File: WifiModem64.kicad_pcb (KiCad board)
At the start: 2 copper layers, 4 parts, among them J1 C64-UserPort, J2 PWR1, U1 WeMos_mini, U2 WeMos_D1_mini_OLED_Shield

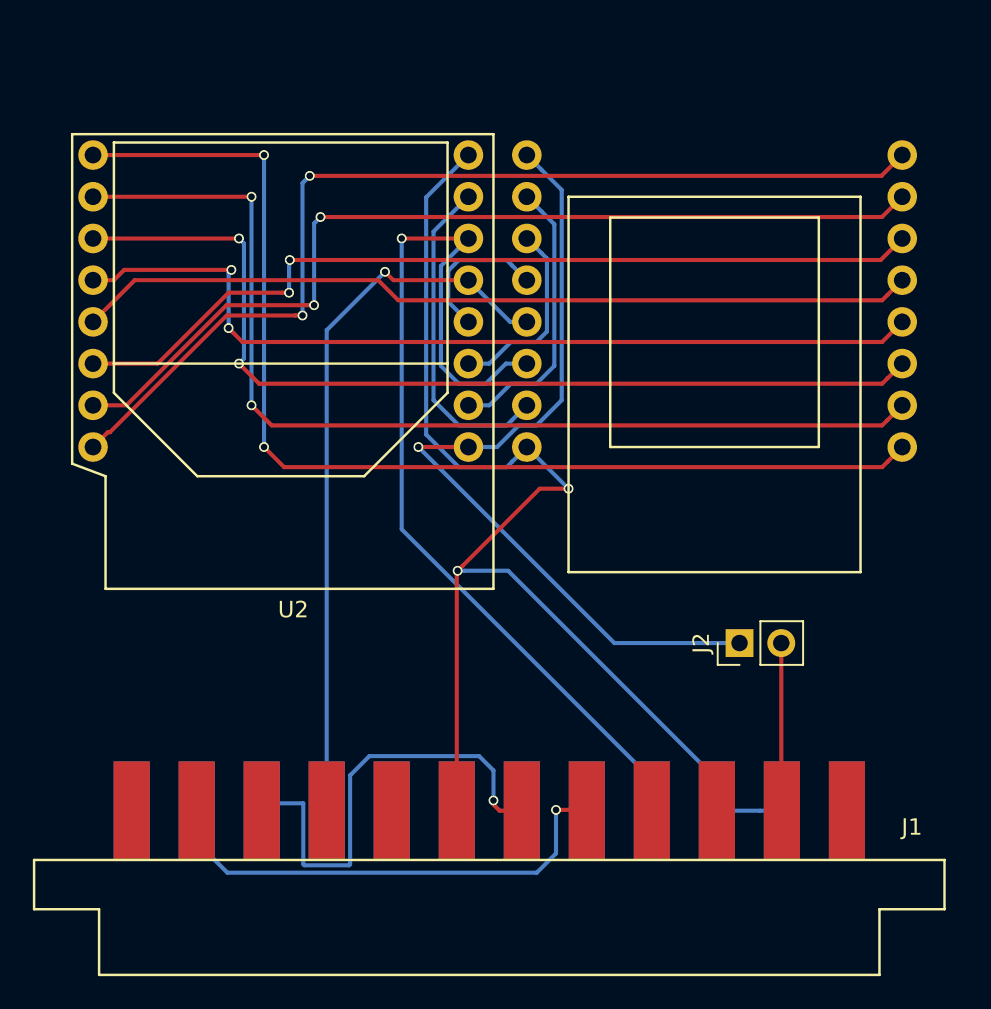
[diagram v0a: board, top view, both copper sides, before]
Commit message: WiP.
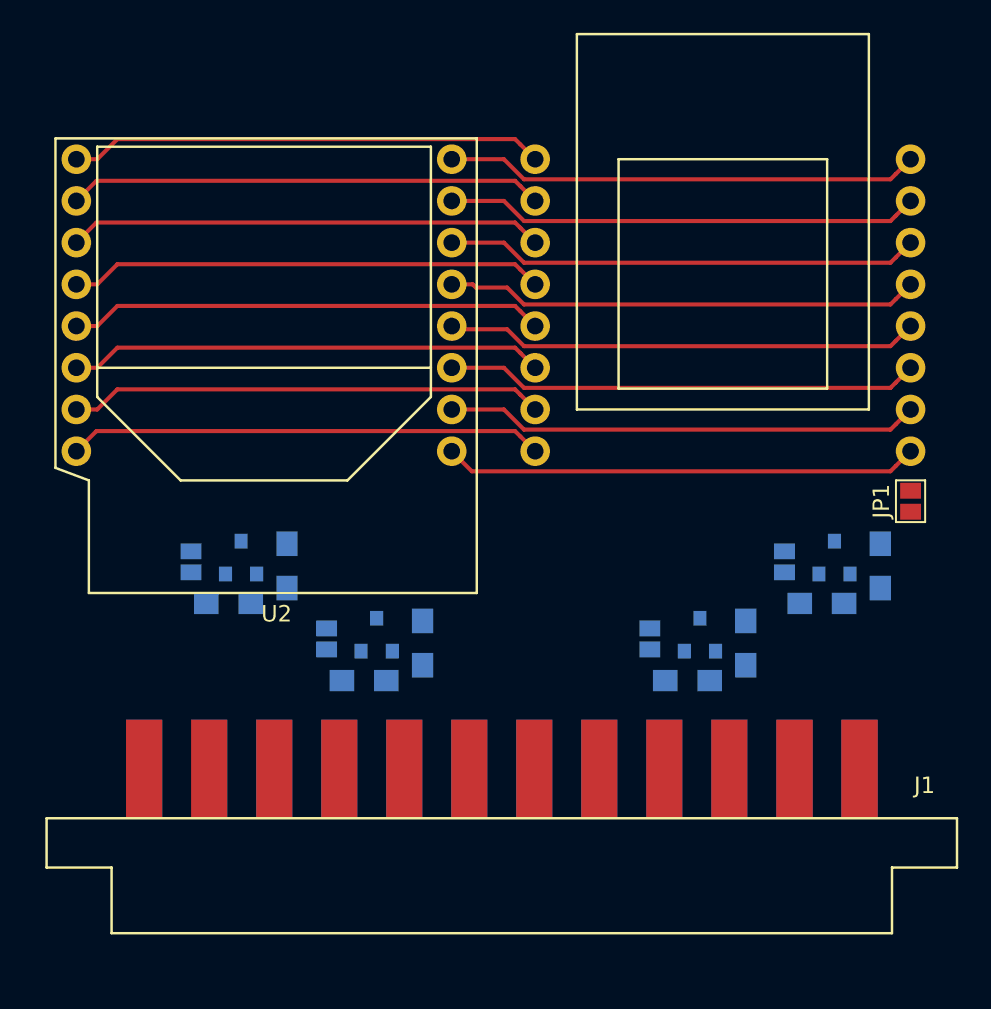
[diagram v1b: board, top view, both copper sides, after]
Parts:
- removed J2: PWR1, Pin_Headers:Pin_Header_Straight_1x02_Pitch2.54mm
- added JP1: IntPwr, Connectors:GS2, F.Cu at (171.4, 105.9)
- added JP2: CTS, Connectors:GS2, B.Cu at (155.6, 114.3)
- added JP3: RTS, Connectors:GS2, B.Cu at (135.9, 114.3)
- added JP4: SP1, Connectors:GS2, B.Cu at (127.6, 109.6)
- added JP5: SP2, Connectors:GS2, B.Cu at (163.8, 109.6)
- added Q1: BSS138, TO_SOT_Packages_SMD:SOT-23, B.Cu at (158.6, 114.0)
- added Q2: BSS138, TO_SOT_Packages_SMD:SOT-23, B.Cu at (138.9, 114.0)
- added Q3: BSS138, TO_SOT_Packages_SMD:SOT-23, B.Cu at (130.7, 109.3)
- added Q4: BSS138, TO_SOT_Packages_SMD:SOT-23, B.Cu at (166.8, 109.3)
- added R1: 10k, Resistors_SMD:R_0805_HandSoldering, B.Cu at (157.9, 116.8)
- added R2: 10k, Resistors_SMD:R_0805_HandSoldering, B.Cu at (138.2, 116.8)
- added R3: 10k, Resistors_SMD:R_0805_HandSoldering, B.Cu at (129.9, 112.1)
- added R4: 10k, Resistors_SMD:R_0805_HandSoldering, B.Cu at (166.1, 112.1)
- added R5: 10k, Resistors_SMD:R_0805_HandSoldering, B.Cu at (161.4, 114.6)
- added R6: 10k, Resistors_SMD:R_0805_HandSoldering, B.Cu at (141.7, 114.6)
- added R7: 10k, Resistors_SMD:R_0805_HandSoldering, B.Cu at (133.5, 109.9)
- added R8: 10k, Resistors_SMD:R_0805_HandSoldering, B.Cu at (169.6, 109.9)
- moved U2 5.59 mm to (132.1, 95.2)
- moved U1 2.84 mm to (160.0, 95.2), turned to 180 degrees
- moved J1 2.65 mm to (146.6, 125.2)
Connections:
- net W_3V3 renamed +3V3
- net W_5V renamed +5V
- net W_GND renamed GND
- J1 pad 5: W_RX -> SP1
- J1 pad 7: W_TX -> SP2
- J1 pad B: W_TX -> SP2
- J1 pad C: W_TX -> SP2
- J1 pad D: W_D1 -> CTS
- J1 pad K: W_D2 -> RTS
- J1 pad M: W_RX -> SP1
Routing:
- net W_TX: track 79.5 -> 29.0 mm, vias 3 -> 0
- net W_RST: track 68.1 -> 29.0 mm, vias 2 -> 0
- net W_A0: track 63.0 -> 29.0 mm, vias 2 -> 0
- net +3V3: track 61.4 -> 29.0 mm, vias 2 -> 0
- net W_D1: track 59.9 -> 29.0 mm, vias 1 -> 0
- net W_D0: track 58.2 -> 29.0 mm, vias 2 -> 0
- net W_D8: track 57.5 -> 29.0 mm, vias 2 -> 0
- net Net-(J1-Pad6): track 28.3 -> 0.00 mm, vias 1 -> 0
- net W_D5: track 54.2 -> 29.0 mm, vias 2 -> 0
- net W_D7: track 53.6 -> 29.0 mm, vias 2 -> 0
- net W_D6: track 51.3 -> 29.0 mm
- net +5V: track 50.2 -> 29.0 mm, vias 1 -> 0
- net W_RX: track 49.7 -> 29.0 mm, vias 1 -> 0
- net W_D3: track 9.19 -> 29.0 mm
- net W_D4: track 11.8 -> 29.0 mm
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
